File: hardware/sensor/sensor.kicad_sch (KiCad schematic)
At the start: 1 part

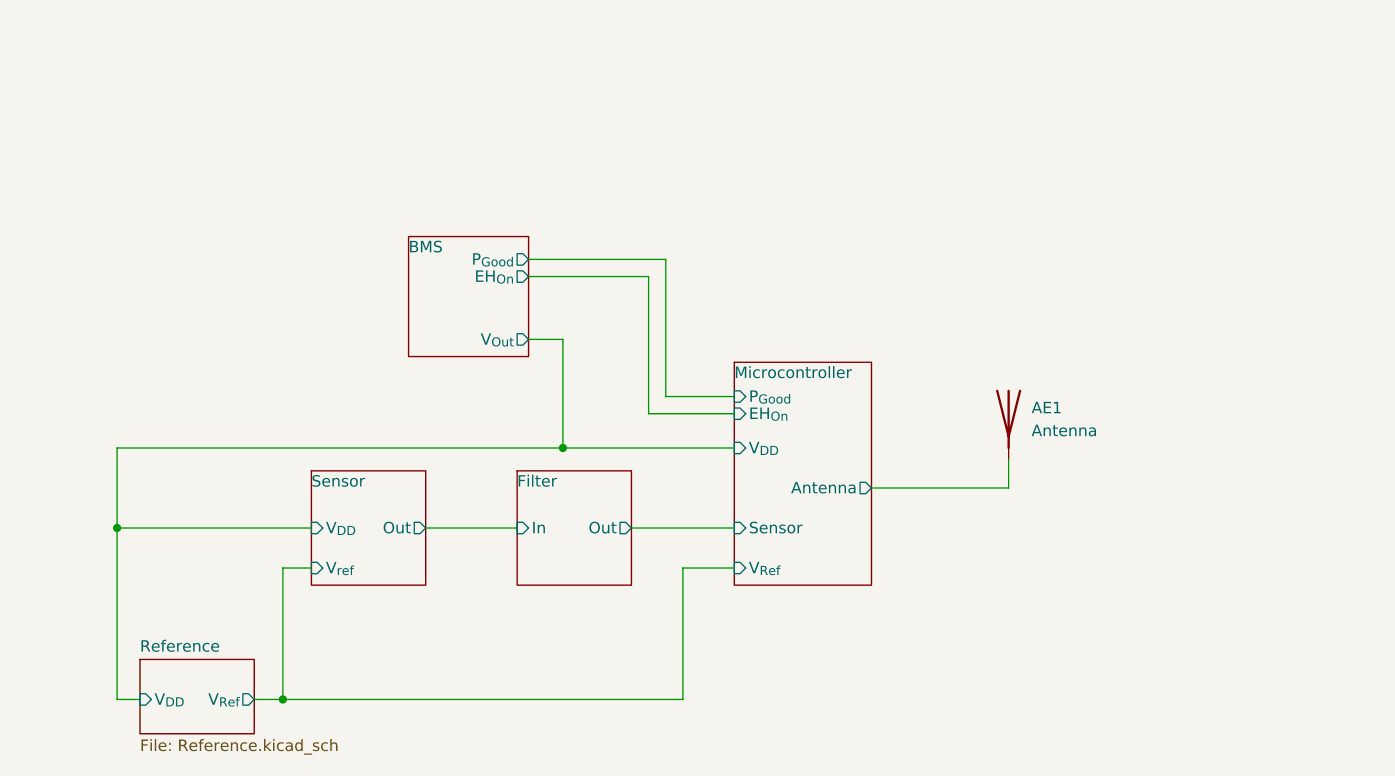
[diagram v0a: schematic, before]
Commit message: commit to save work from misbehaving laptop
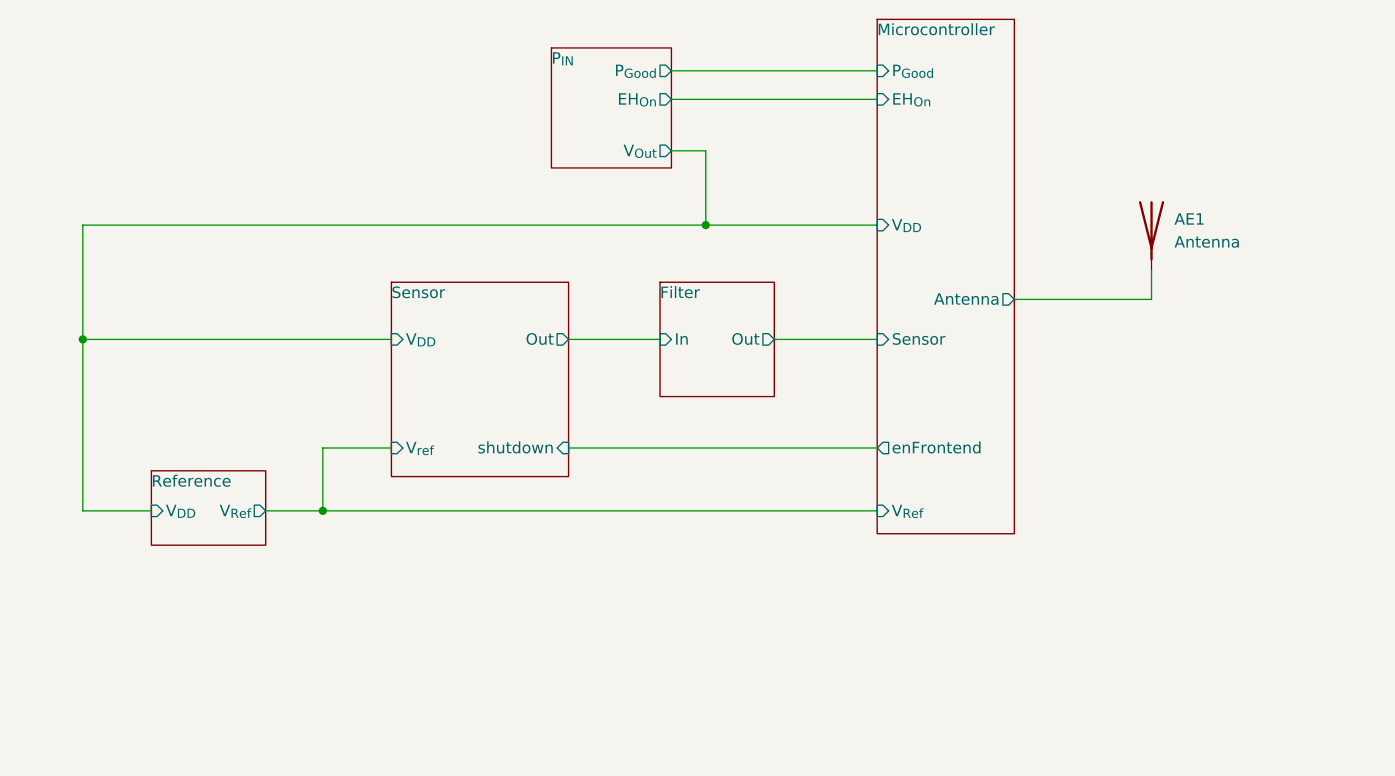
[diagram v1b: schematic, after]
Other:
- sheet BMS renamed P_{IN}
- sheet Microcontroller ports: added enFrontend; removed none
- sheet Sensor ports: added shutdown; removed none
- moved on the sheet: AE1

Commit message: Fix incorrect upstream
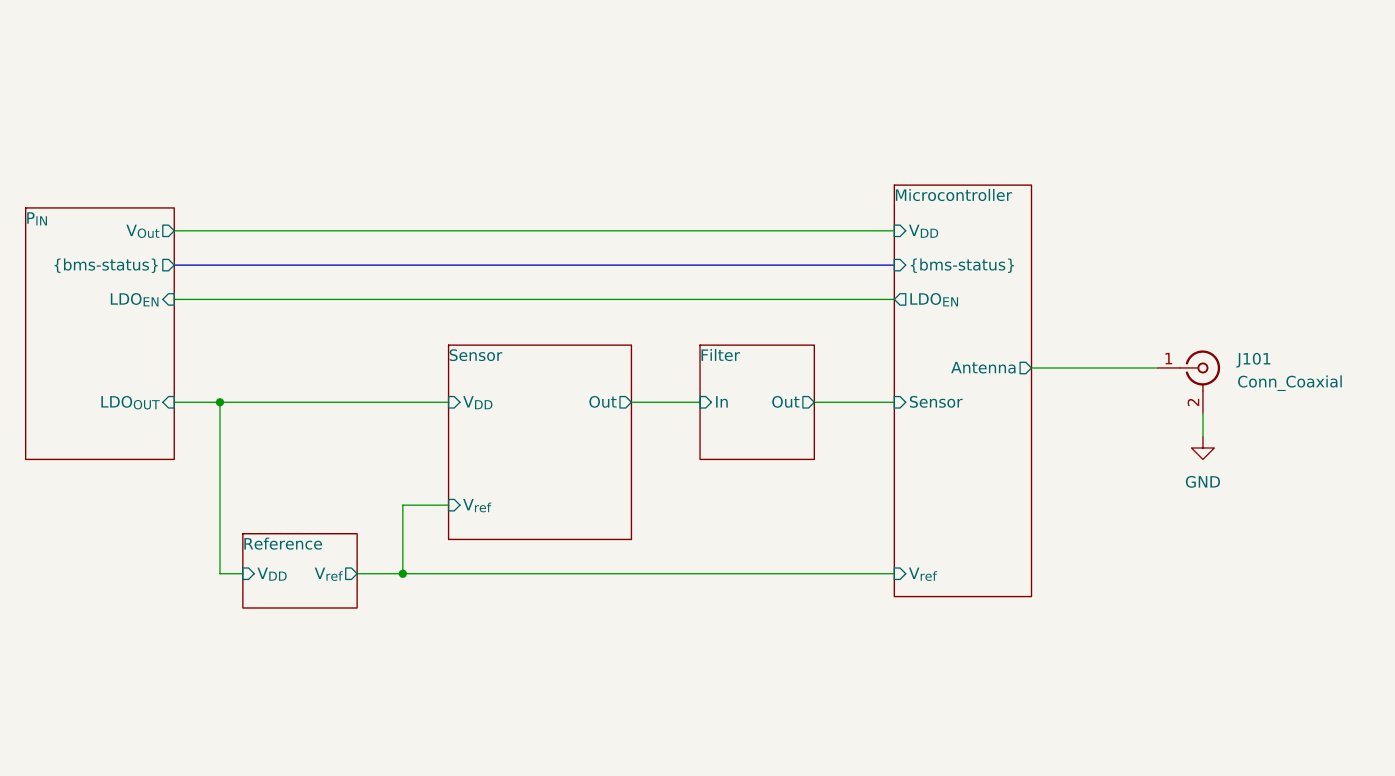
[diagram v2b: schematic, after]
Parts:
- removed AE1: Antenna, symbol Device:Antenna
- added J101: Conn_Coaxial, Connector_Coaxial:SMA_Amphenol_901-143_Horizontal, symbol Connector:Conn_Coaxial
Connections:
- net Microcontroller/Antenna: now also J101.1 (In)
- new net GND: J101.2 (Ext)
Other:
- sheet Microcontroller ports: added LDO_{EN}, V_{ref}, {bms-status}; removed EH_{On}, P_{Good}, V_{Ref}, enFrontend
- sheet P_{IN} ports: added LDO_{EN}, LDO_{OUT}, {bms-status}; removed EH_{On}, P_{Good}
- sheet Reference ports: added V_{ref}; removed V_{Ref}
- sheet Sensor ports: added none; removed shutdown
